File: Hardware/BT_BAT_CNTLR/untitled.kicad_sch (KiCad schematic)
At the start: 9 parts, among them J2 USB_A, U4 AP22814AW5, U5 SN74LVC1T45DRL

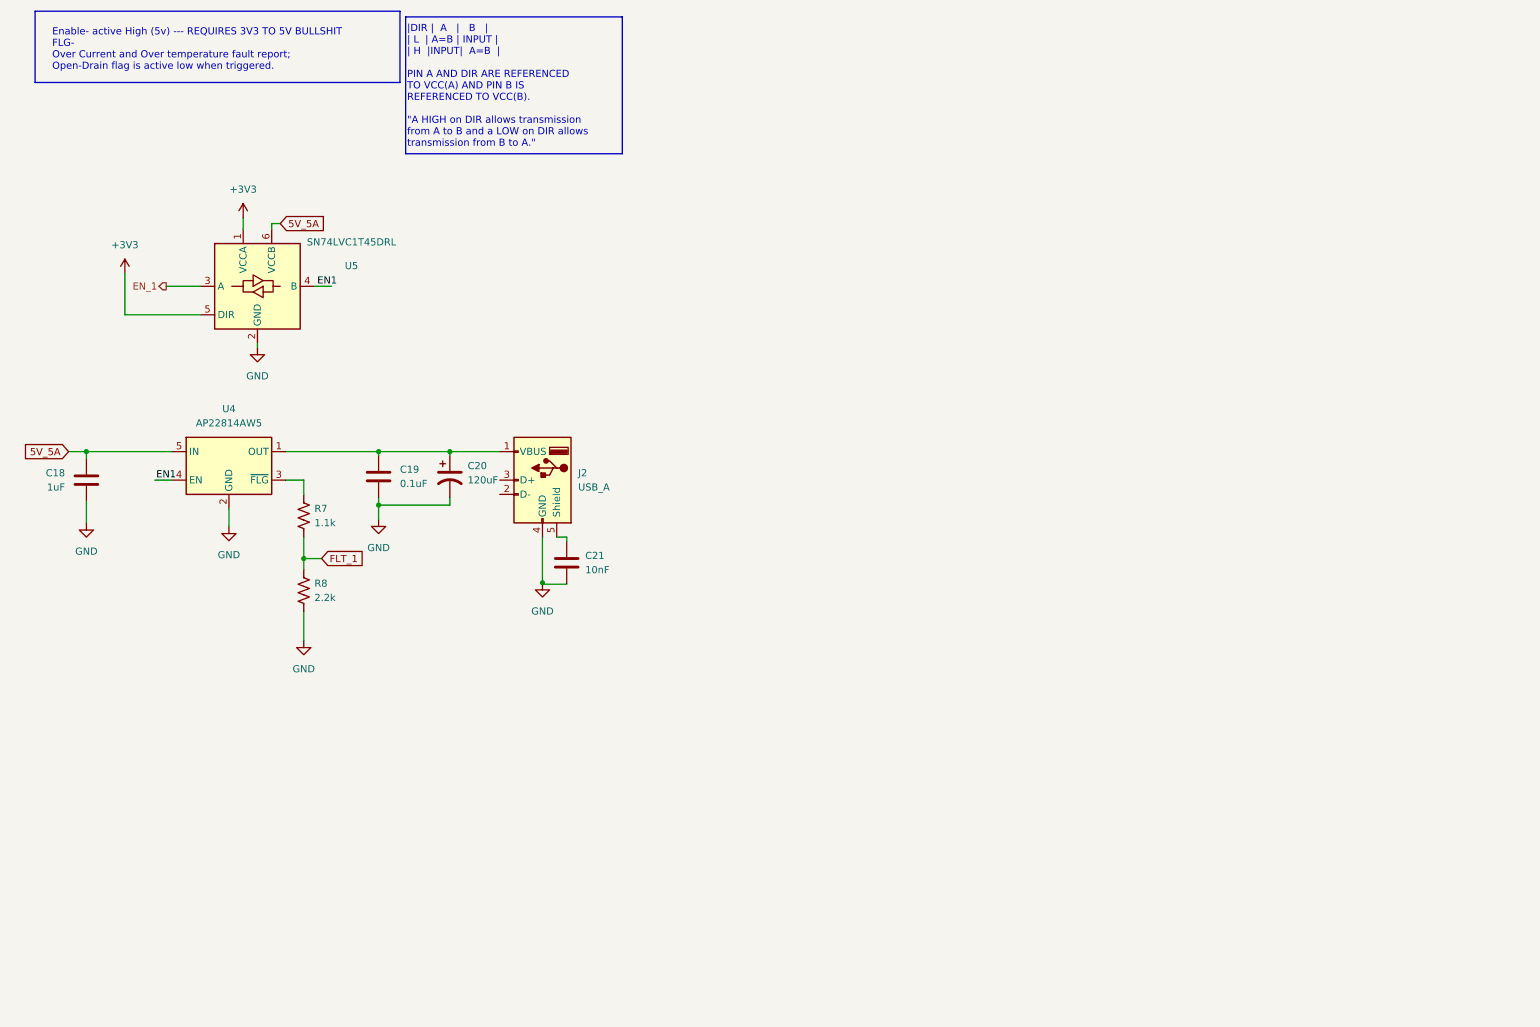
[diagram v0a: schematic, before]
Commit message: - Github Tree Cleanup - Power Routing
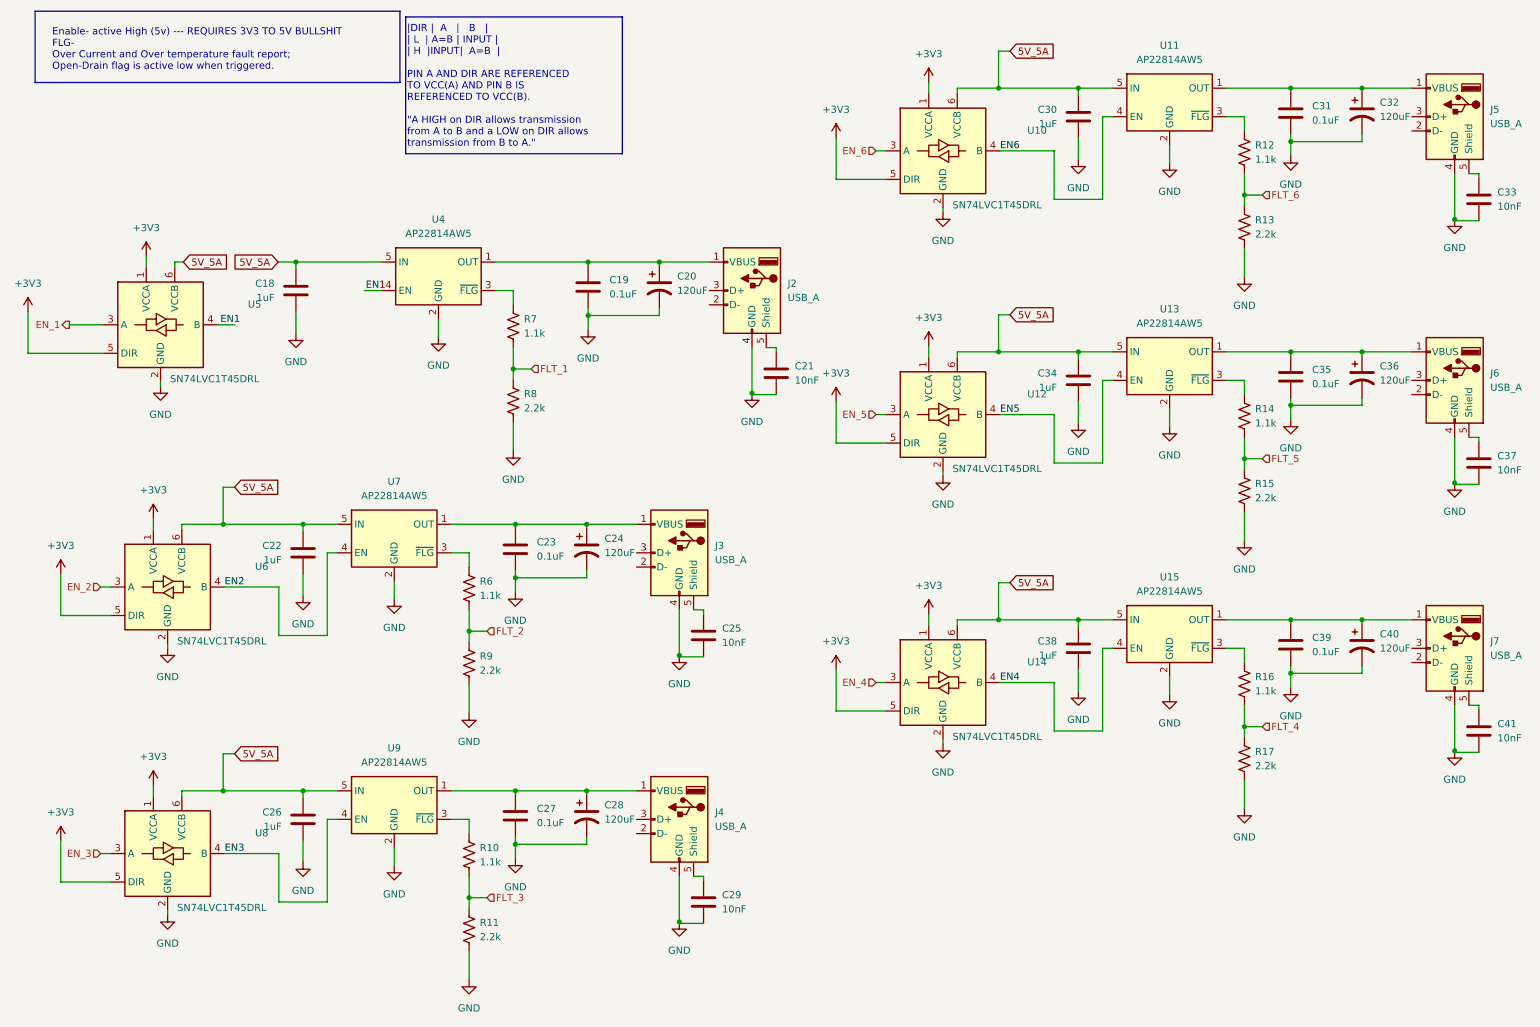
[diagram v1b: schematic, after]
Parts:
- added C22, C26, C30, C34, C38: 1uF, Capacitor_SMD:C_0603_1608Metric, symbol Device:C
- added C23, C27, C31, C35, C39: 0.1uF, Capacitor_SMD:C_0603_1608Metric, symbol Device:C
- added C24, C28, C32, C36, C40: 120uF, Capacitor_SMD:CP_Elec_5x5.9, symbol Device:C_Polarized_US
- added C25, C29, C33, C37, C41: 10nF, Capacitor_SMD:C_0603_1608Metric, symbol Device:C
- added J3, J4, J5, J6, J7: USB_A, Connector_USB:USB_A_Molex_67643_Horizontal, symbol Connector:USB_A
- added R10, R12, R14, R16, R6: 1.1k, Resistor_SMD:R_0603_1608Metric, symbol Device:R_US
- added R11, R13, R15, R17, R9: 2.2k, Resistor_SMD:R_0603_1608Metric, symbol Device:R_US
- added U10, U12, U14, U6, U8: SN74LVC1T45DRL, Package_TO_SOT_SMD:SOT-563, symbol Logic_LevelTranslator:SN74LVC1T45DRL
- added U11, U13, U15, U7, U9: AP22814AW5, Package_TO_SOT_SMD:SOT-23-5, symbol Power_Management:AP22814AW5
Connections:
- net +3V3: now also U10.1 (VCCA), U10.5 (DIR), U12.1 (VCCA), U12.5 (DIR), U14.1 (VCCA), U14.5 (DIR), U6.1 (VCCA), U6.5 (DIR), U8.1 (VCCA), U8.5 (DIR)
- net 5V_5A: now also C22.1, C26.1, C30.1, C34.1, C38.1, U10.6 (VCCB), U11.5 (IN), U12.6 (VCCB), U13.5 (IN), U14.6 (VCCB), U15.5 (IN), U6.6 (VCCB), U7.5 (IN), U8.6 (VCCB), U9.5 (IN)
- net GND: now also C22.2, C23.2, C24.2, C25.2, C26.2, C27.2, C28.2, C29.2, C30.2, C31.2, C32.2, C33.2, C34.2, C35.2, C36.2, C37.2, C38.2, C39.2, C40.2, C41.2, J3.4 (GND), J4.4 (GND), J5.4 (GND), J6.4 (GND), J7.4 (GND), R11.2, R13.2, R15.2, R17.2, R9.2, U10.2 (GND), U11.2 (GND), U12.2 (GND), U13.2 (GND), U14.2 (GND), U15.2 (GND), U6.2 (GND), U7.2 (GND), U8.2 (GND), U9.2 (GND)
- new net: C27.1, C28.1, J4.1 (VBUS), U9.1 (OUT)
- new net: C35.1, C36.1, J6.1 (VBUS), U13.1 (OUT)
- new net: C31.1, C32.1, J5.1 (VBUS), U11.1 (OUT)
- new net: C33.1, J5.5 (Shield)
- new net: C29.1, J4.5 (Shield)
- new net: C39.1, C40.1, J7.1 (VBUS), U15.1 (OUT)
- new net: R12.1, U11.3 (~{FLG})
- new net: C25.1, J3.5 (Shield)
- new net: R16.1, U15.3 (~{FLG})
- new net: C37.1, J6.5 (Shield)
- new net: C23.1, C24.1, J3.1 (VBUS), U7.1 (OUT)
- new net: R10.1, U9.3 (~{FLG})
- new net: R6.1, U7.3 (~{FLG})
- new net: C41.1, J7.5 (Shield)
- new net: R14.1, U13.3 (~{FLG})
- new net EN2: U6.4 (B), U7.4 (EN)
- new net EN3: U8.4 (B), U9.4 (EN)
- new net EN4: U14.4 (B), U15.4 (EN)
- new net EN5: U12.4 (B), U13.4 (EN)
- new net EN6: U10.4 (B), U11.4 (EN)
- new net EN_2: U6.3 (A)
- new net EN_3: U8.3 (A)
- new net EN_4: U14.3 (A)
- new net EN_5: U12.3 (A)
- new net EN_6: U10.3 (A)
- new net FLT_2: R6.2, R9.1
- new net FLT_3: R10.2, R11.1
- new net FLT_4: R16.2, R17.1
- new net FLT_5: R14.2, R15.1
- new net FLT_6: R12.2, R13.1
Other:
- moved on the sheet: C18, C19, C20, C21, J2, R7, R8, U4, U5
